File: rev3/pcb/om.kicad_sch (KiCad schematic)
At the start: 44 parts, among them J1 USB_C_Receptacle, J2 JST-BATT, J4 SWD, Q1 AO3407, Q2 AO3407, SW1 Choc, SW10 Choc, SW11 Choc, SW12 Choc, SW13 Choc, SW14 Choc, SW15 Choc, SW16 Choc, SW17 Choc, SW2 Choc, SW3 Choc, SW4 Choc, SW5 Choc, SW6 Choc, SW7 Choc, SW8 Choc, SW9 Choc, U1 nRF52840_holyiot_18010, U2 XC6206P LDO, U3 LTC4054ES5-4.2

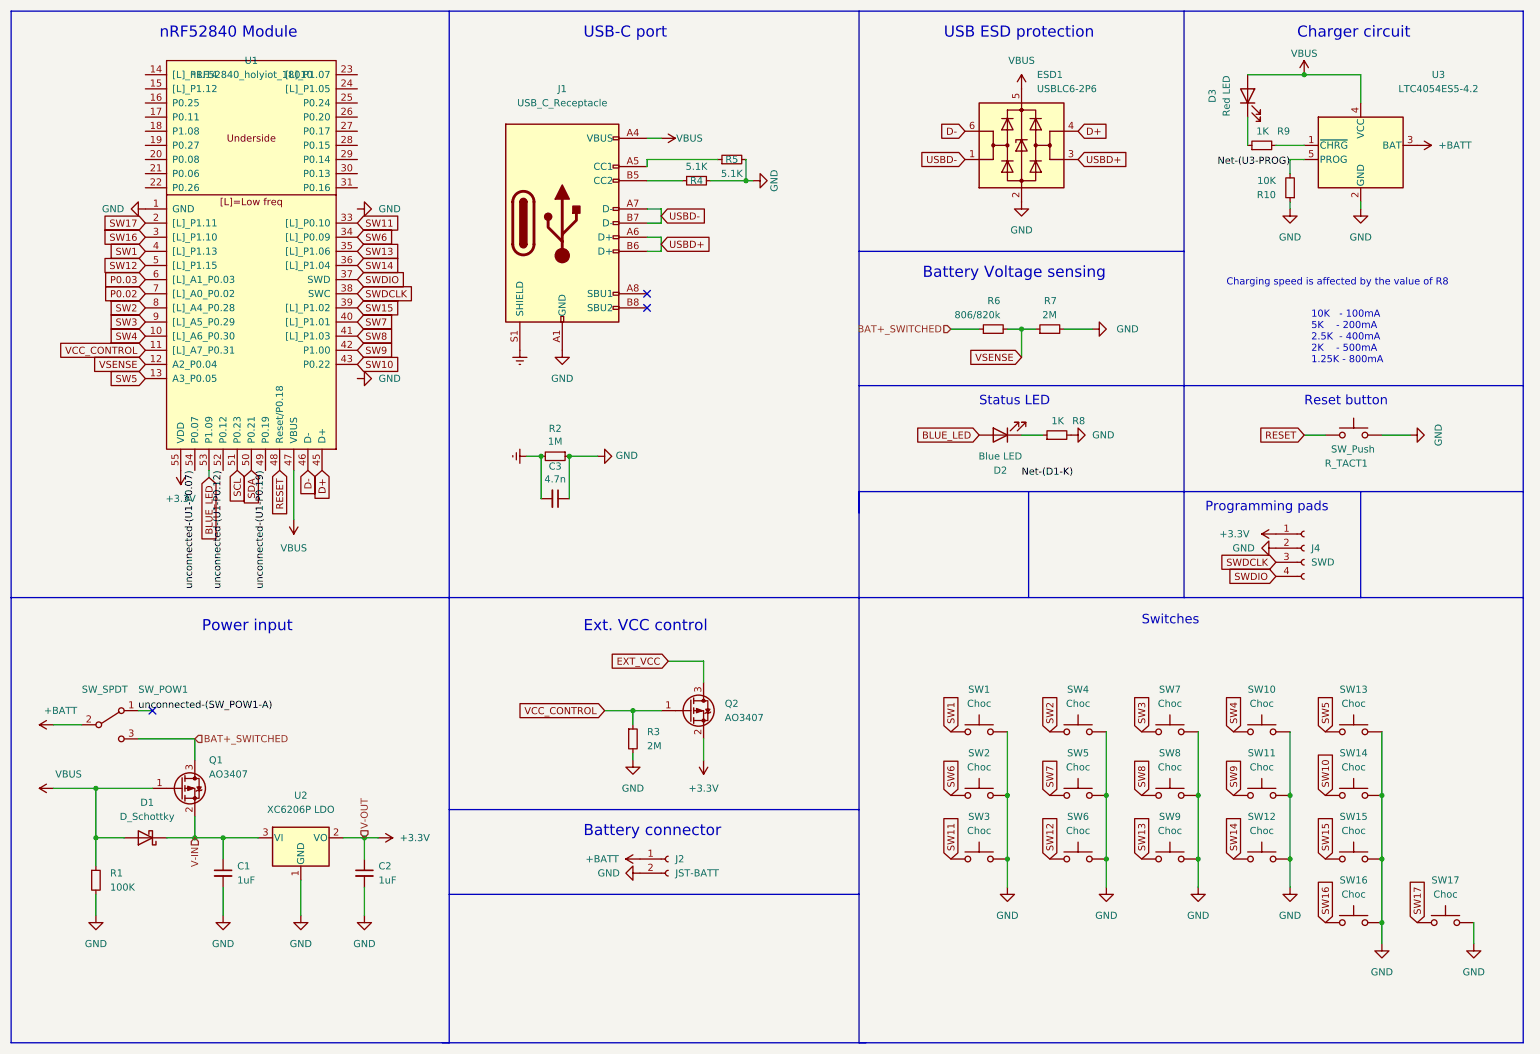
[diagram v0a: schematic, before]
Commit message: Routing might be done?
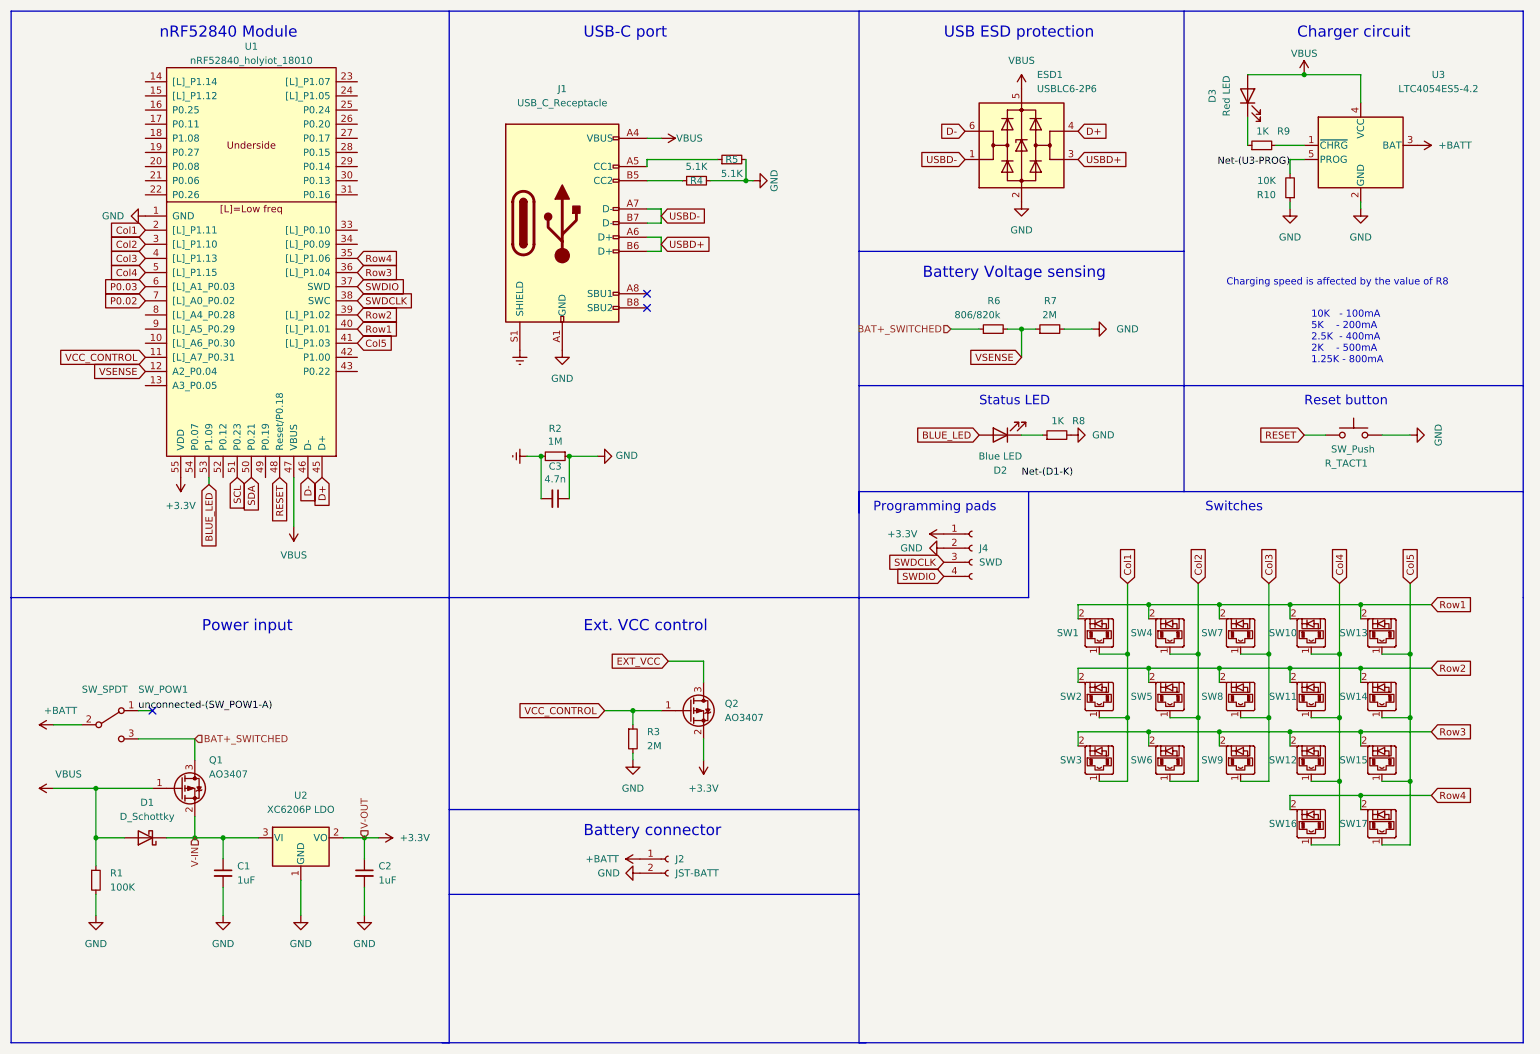
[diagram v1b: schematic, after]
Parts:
- R_TACT1: footprint Button_Switch_SMD:SW_SPST_TL3342 -> om-footprints:SKHLLCA010
- SW1, SW10, SW11, SW12, SW13, SW14, SW15, SW16, SW17, SW2, SW3, SW4, SW5, SW6, SW7, SW8, SW9: footprint kleeb-pg1350:pg1350-R -> kleeb-pg1350:pg1350-DR; symbol Switch:SW_Push -> kleeb-switches:diode-choc
- U1: footprint mcu:holyiot-18010 -> kleeb-mcu:holyiot-18010
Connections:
- net GND: no longer SW1.2, SW10.2, SW11.2, SW12.2, SW13.2, SW14.2, SW15.2, SW16.2, SW17.2, SW2.2, SW3.2, SW4.2, SW5.2, SW6.2, SW7.2, SW8.2, SW9.2
- net SW1 renamed Col1
- net Col1: now also SW2.1, SW3.1, U1.2 ([L]_P1.11); no longer U1.4 ([L]_P1.13)
- net SW10: no longer names the net of U1.43 (P0.22)
- net SW10: no longer SW14.1
- net SW11: no longer names the net of U1.33 ([L]_P0.10)
- net SW11: no longer SW3.1
- net SW12 renamed Col2
- net Col2: now also SW4.1, SW5.1, U1.3 ([L]_P1.10); no longer U1.5 ([L]_P1.15)
- net SW13 renamed Col3
- net Col3: now also SW7.1, SW8.1, U1.4 ([L]_P1.13); no longer U1.35 ([L]_P1.06)
- net SW14 renamed Col4
- net Col4: now also SW10.1, SW11.1, SW16.1, U1.5 ([L]_P1.15); no longer U1.36 ([L]_P1.04)
- net SW15 renamed Col5
- net Col5: now also SW13.1, SW14.1, SW17.1, U1.41 ([L]_P1.03); no longer U1.39 ([L]_P1.02)
- removed net SW16: SW16.1, U1.3 ([L]_P1.10)
- removed net SW17: SW17.1, U1.2 ([L]_P1.11)
- net SW2: no longer names the net of U1.8 ([L]_A4_P0.28)
- net SW2: no longer SW4.1
- net SW3: no longer names the net of U1.9 ([L]_A5_P0.29)
- net SW3: no longer SW7.1
- net SW4: no longer names the net of U1.10 ([L]_A6_P0.30)
- net SW4: no longer SW10.1
- net SW5: no longer names the net of U1.13 (A3_P0.05)
- net SW5: no longer SW13.1
- net SW6: no longer names the net of U1.34 ([L]_P0.09)
- net SW6: no longer SW2.1
- net SW7 renamed Row1
- net Row1: now also SW1.2, SW10.2, SW13.2, SW4.2, SW7.2; no longer SW5.1
- removed net SW8: SW8.1, U1.41 ([L]_P1.03)
- net SW9: no longer names the net of U1.42 (P1.00)
- net SW9: no longer SW11.1
- net unconnected-(U1-P0.07): no longer names the net of U1.54 (P0.07)
- net unconnected-(U1-P0.12): no longer names the net of U1.52 (P0.12)
- net unconnected-(U1-P0.19): no longer names the net of U1.49 (P0.19)
- new net Row2: SW11.2, SW14.2, SW2.2, SW5.2, SW8.2, U1.39 ([L]_P1.02)
- new net Row3: SW12.2, SW15.2, SW3.2, SW6.2, SW9.2, U1.36 ([L]_P1.04)
- new net Row4: SW16.2, SW17.2, U1.35 ([L]_P1.06)
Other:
- moved on the sheet: J4, U1

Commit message: Mostly in place, time to refactor
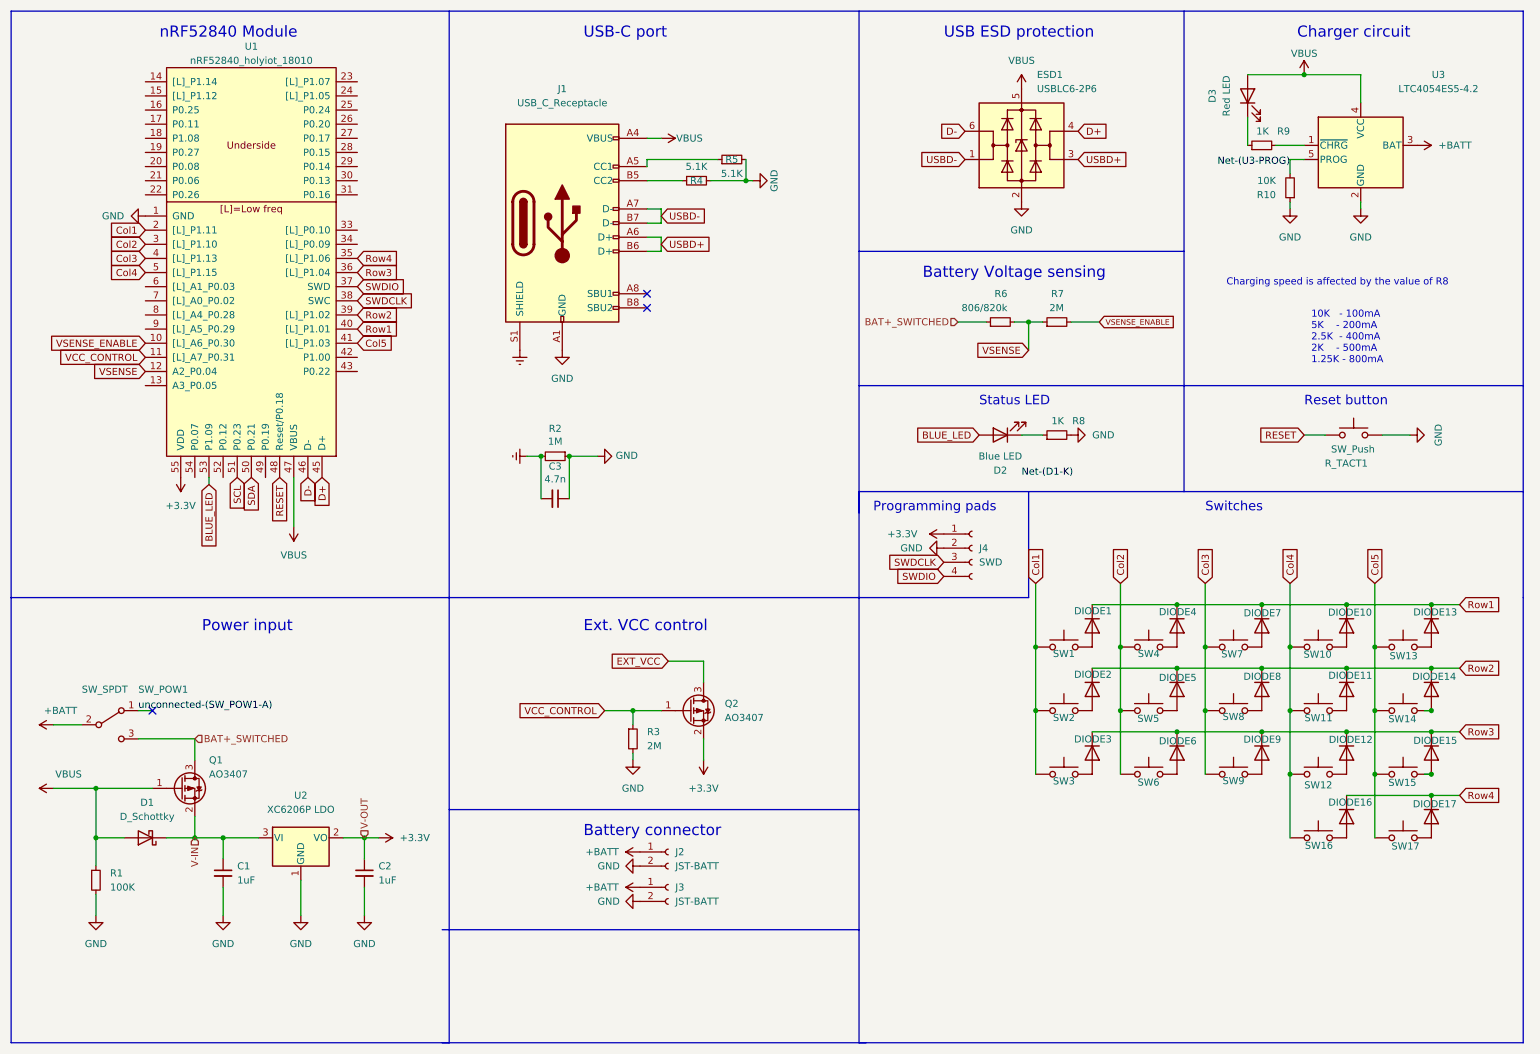
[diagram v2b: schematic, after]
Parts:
- added DIODE1, DIODE10, DIODE11, DIODE12, DIODE13, DIODE14, DIODE15, DIODE16, DIODE17, DIODE2, DIODE3, DIODE4, DIODE5, DIODE6, DIODE7, DIODE8, DIODE9: 1N914WT, Diode_SMD:D_SOD-123, symbol Diode:1N914WT
- added J3: JST-BATT, Connector_JST:JST_PH_S2B-PH-K_1x02_P2.00mm_Horizontal, symbol Connector:Conn_01x02_Female
- C1, C2: LCSC (none) -> C15849
- C3: LCSC (none) -> C1744
- D1: LCSC (none) -> C191023
- R_TACT1: LCSC (none) -> C139766
- SW1, SW10, SW11, SW12, SW13, SW14, SW15, SW16, SW17, SW2, SW3, SW4, SW5, SW6, SW7, SW8, SW9: footprint kleeb-pg1350:pg1350-DR -> kleeb-pg1350:pg1350; symbol kleeb-switches:diode-choc -> Switch:SW_Push
- U3: LCSC (none) -> C462648
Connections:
- net +BATT: now also J3.1 (Pin_1)
- net GND: now also J3.2 (Pin_2); no longer R7.2
- net Row1: now also DIODE1.1 (K), DIODE10.1 (K), DIODE13.1 (K), DIODE4.1 (K), DIODE7.1 (K); no longer SW1.2, SW10.2, SW13.2, SW4.2, SW7.2
- net Row2: now also DIODE11.1 (K), DIODE14.1 (K), DIODE2.1 (K), DIODE5.1 (K), DIODE8.1 (K); no longer SW11.2, SW14.2, SW2.2, SW5.2, SW8.2
- net Row3: now also DIODE12.1 (K), DIODE15.1 (K), DIODE3.1 (K), DIODE6.1 (K), DIODE9.1 (K); no longer SW12.2, SW15.2, SW3.2, SW6.2, SW9.2
- net Row4: now also DIODE16.1 (K), DIODE17.1 (K); no longer SW16.2, SW17.2
- net VSENSE_ENABLE: now reaches U1.10 ([L]_A6_P0.30)
- net VSENSE_ENABLE: now also R7.2
- net P0.02: no longer names the net of U1.7 ([L]_A0_P0.02)
- net P0.03: no longer names the net of U1.6 ([L]_A1_P0.03)
- new net: DIODE9.2 (A), SW9.2
- new net: DIODE4.2 (A), SW4.2
- new net: DIODE5.2 (A), SW5.2
- new net: DIODE15.2 (A), SW15.2
- new net: DIODE13.2 (A), SW13.2
- new net: DIODE16.2 (A), SW16.2
- new net: DIODE1.2 (A), SW1.2
- new net: DIODE17.2 (A), SW17.2
- new net: DIODE3.2 (A), SW3.2
- new net: DIODE2.2 (A), SW2.2
- new net: DIODE7.2 (A), SW7.2
- new net: DIODE11.2 (A), SW11.2
- new net: DIODE12.2 (A), SW12.2
- new net: DIODE8.2 (A), SW8.2
- new net: DIODE6.2 (A), SW6.2
- new net: DIODE14.2 (A), SW14.2
- new net: DIODE10.2 (A), SW10.2
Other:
- moved on the sheet: J2, R6, R7
